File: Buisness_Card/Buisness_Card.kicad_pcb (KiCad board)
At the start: 2 copper layers, 85.6 x 53.9 mm, 3 parts, among them IC1 NT2H1311F0DTL

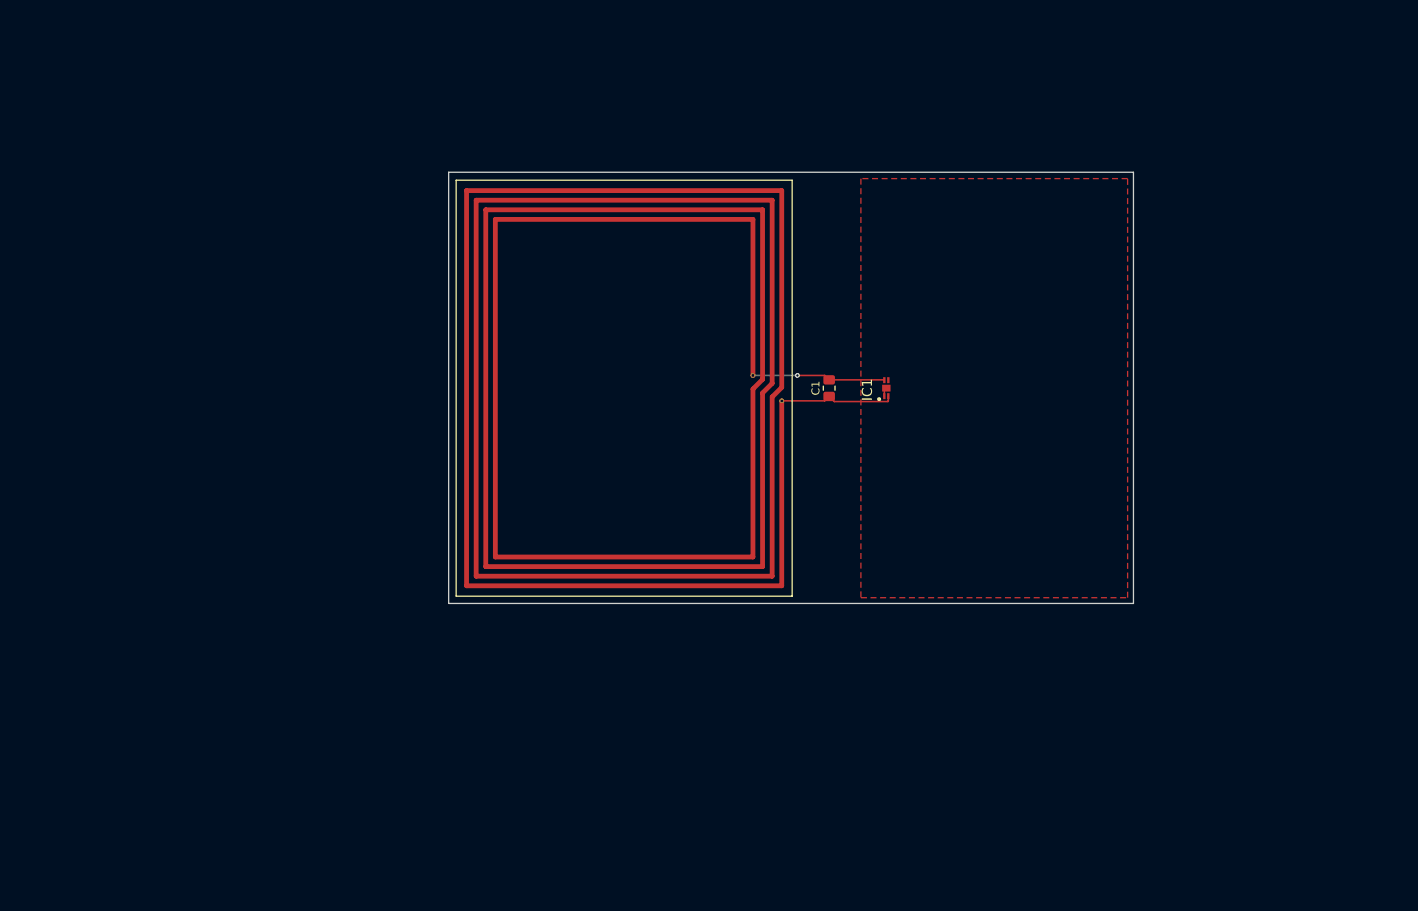
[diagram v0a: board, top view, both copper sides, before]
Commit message: finish :)
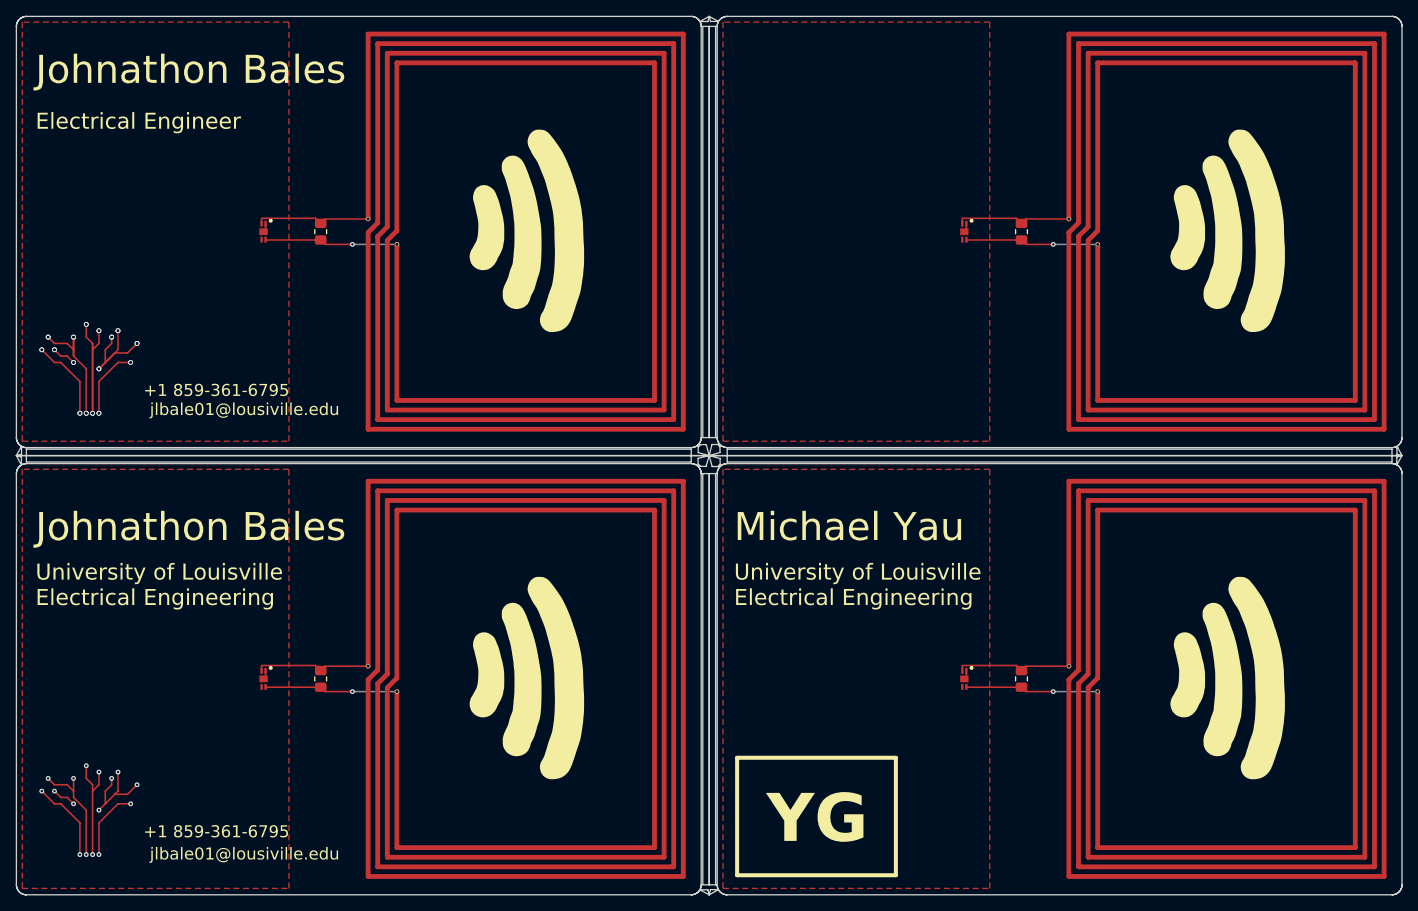
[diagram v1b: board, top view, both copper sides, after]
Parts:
- removed the ANT1 at (116.3, 105.2)
- removed the C1 at (161.9, 80.2)
- removed the IC1 at (169.1, 80.2)
- added ANT1: 2.69uH, nfc_ant:BANTnfcv2, F.Cu at (231.6, 35.6)
- added ANT1: 2.69uH, nfc_ant:BANTnfcv2, F.Cu at (144.0, 91.5)
- added ANT1: 2.69uH, nfc_ant:BANTnfcv2, F.Cu at (144.0, 35.6)
- added ANT1: 2.69uH, nfc_ant:BANTnfcv2, F.Cu at (231.6, 91.5)
- added C1: 1.2pF, Capacitor_SMD:C_0805_2012Metric_Pad1.18x1.45mm_HandSolder, F.Cu at (186.0, 116.5)
- added C1: 1.2pF, Capacitor_SMD:C_0805_2012Metric_Pad1.18x1.45mm_HandSolder, F.Cu at (98.4, 60.6)
- added C1: 1.2pF, Capacitor_SMD:C_0805_2012Metric_Pad1.18x1.45mm_HandSolder, F.Cu at (98.4, 116.5)
- added C1: 1.2pF, Capacitor_SMD:C_0805_2012Metric_Pad1.18x1.45mm_HandSolder, F.Cu at (186.0, 60.6)
- added G***: LOGO, LOGO, F.Cu at (211.7, 60.5)
- added G***: LOGO, LOGO, F.Cu at (124.1, 116.4)
- added G***: LOGO, LOGO, F.Cu at (211.7, 116.4)
- added G***: LOGO, LOGO, F.Cu at (124.1, 60.5)
- added G***: LOGO, LOGO, B.Cu at (82.6, 68.6)
- added G***: LOGO, LOGO, B.Cu at (123.8, 60.7)
- added G***: LOGO, LOGO, B.Cu at (123.8, 116.9)
- added G***: LOGO, LOGO, B.Cu at (83.3, 125.0)
- added IC1: NT2H1311F0DTL, temp:SON50P200X150X50-5N, F.Cu at (178.8, 60.6)
- added IC1: NT2H1311F0DTL, temp:SON50P200X150X50-5N, F.Cu at (91.2, 116.5)
- added IC1: NT2H1311F0DTL, temp:SON50P200X150X50-5N, F.Cu at (91.2, 60.6)
- added IC1: NT2H1311F0DTL, temp:SON50P200X150X50-5N, F.Cu at (178.8, 116.5)
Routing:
- net Board_3-GND: track 0.00 -> 141.1 mm, vias 0 -> 48
- net Board_3-LA: track 0.00 -> 16.7 mm, vias 0 -> 1
- net Board_1-LA: track 0.00 -> 16.7 mm, vias 0 -> 1
- net LA: track 16.7 -> 0.00 mm, vias 1 -> 0
- net Board_2-LA: track 0.00 -> 16.7 mm, vias 0 -> 1
- net Board_0-LA: track 0.00 -> 16.7 mm, vias 0 -> 1
- net Board_1-LB: track 0.00 -> 14.5 mm
- net Board_0-LB: track 0.00 -> 14.5 mm
- net LB: track 14.5 -> 0.00 mm
- net Board_3-LB: track 0.00 -> 14.5 mm
- net Board_2-LB: track 0.00 -> 14.5 mm
- net GND: track 1.10 -> 0.00 mm
- net Board_2-GND: track 0.00 -> 1.10 mm
- net Board_1-GND: track 0.00 -> 1.10 mm
- net Board_0-GND: track 0.00 -> 1.10 mm
- added copper zone on F.Cu, net Board_0-GND
- added copper zone on F.Cu, net Board_1-GND
- added copper zone on F.Cu, net Board_2-GND
- added copper zone on F.Cu, net Board_3-GND
- removed copper zone on F.Cu, net GND
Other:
- board size 85.6 x 53.9 mm -> 173.2 x 109.8 mm
- board text added: "+1 502-579-0895"
- board text added: "+1 859-361-6795"
- board text added: "30x30 QR"
- board text added: "Designed by: Johnathon Bales"
- board text added: "Electrical Engineer"
- board text added: "Electrical Engineering"
- board text added: "Johnathon Bales"
- board text added: "Michael Yau"
- board text added: "University of Louisville"
- board text added: "V-CUT"
- board text added: "YG"
- board text added: "gaudingyu.yau@louisville.edu"
- board text added: "jlbale01@lousiville.edu"
